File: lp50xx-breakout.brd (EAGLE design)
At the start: 31.8 x 29.2 mm, 17 parts, among them U1 LP5024

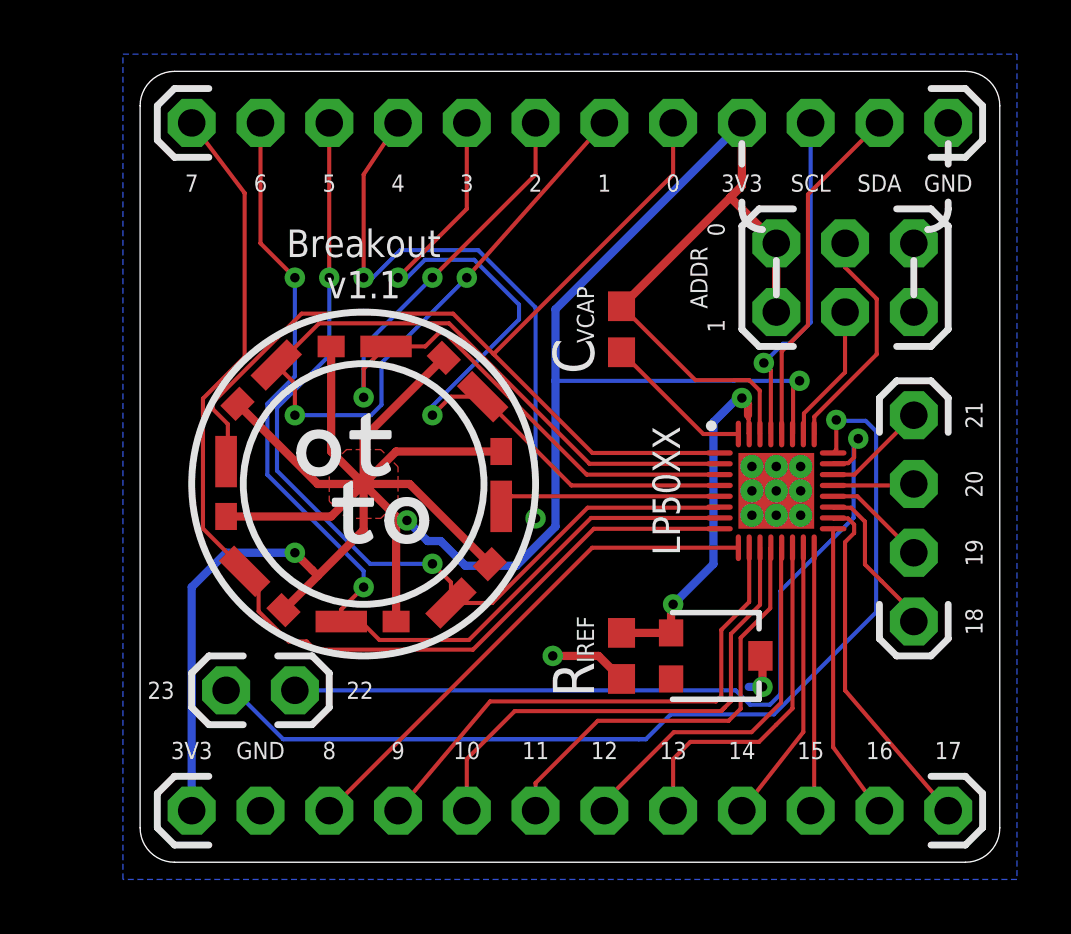
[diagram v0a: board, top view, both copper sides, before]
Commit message: Update design
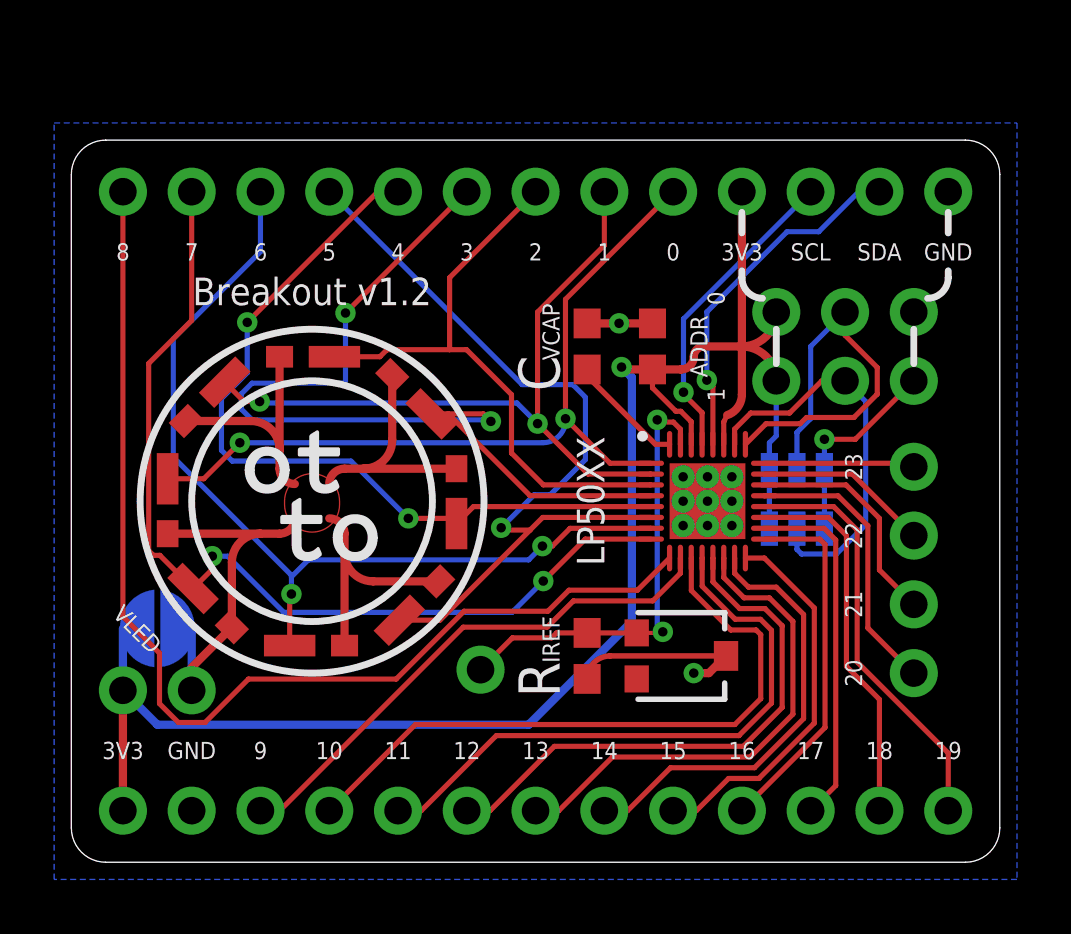
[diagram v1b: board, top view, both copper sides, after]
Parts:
- added C1: 1.0uF, SparkFun-Capacitors:0603
- added JP6: JUMPER-SMT_2_NO_NO-SILK_ROUND, SparkFun-Jumpers:SMT-JUMPER_2_NO_NO-SILK_ROUND
- added JP7, JP8: JUMPER-SMT_3_NO_NO_SILK, SparkFun-Jumpers:SMT-JUMPER_3_0-NO_TRACE_NO-SILK
- added JP9: (no value), pinhead-otto:1X01
- D1, D2, D3, D4, D5, D6, D7, D8: value (none) -> White, 60mA
- JP1, JP2: device pinhead-otto:1X12 -> pinhead-otto:1X13
- moved JP5 3.81 mm to (0.64, 6.35)
- moved JP1 2.84 mm to (14.6, 24.8)
- moved U1 2.57 mm to (21.0, 13.3)
- moved JP3 2.54 mm to (26.0, 19.1)
- moved D1 2.25 mm to (1.02, 13.3)
- moved D7 2.10 mm to (6.35, 8.00)
- moved D2 2.01 mm to (2.54, 17.1)
- moved D4 2.01 mm to (10.2, 17.1)
- moved D8 2.01 mm to (2.54, 9.53)
- moved D6 2.01 mm to (10.2, 9.53)
- moved D3 1.94 mm to (6.35, 18.7)
- moved JP4 1.90 mm to (28.6, 10.8), turned to 270 degrees
- moved D5 1.77 mm to (11.7, 13.3)
- moved C_VCAP 1.42 mm to (16.5, 19.1)
- moved JP2 1.27 mm to (14.6, 1.91)
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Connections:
- net N$5 renamed VCAP
- removed net N$1: R_IREF.2, U1.31, VR1.1
- new net IREF: JP9.1, R_IREF.2, U1.31, VR1.1
- new net VCC: D1.A, D2.A, D3.A, D4.A, D5.A, D6.A, D7.A, D8.A, JP5.1, JP6.2
- net +3V3: now also C1.1, JP5.2, JP6.1, JP7.3, JP8.1; no longer C_VCAP.1, D1.A, D2.A, D3.A, D4.A, D5.A, D6.A, D7.A, D8.A
- net ADDR0: now also JP8.2
- net ADDR1: now also JP7.2
- net GND: now also C1.2, C_VCAP.1, JP7.1, JP8.3
- net OUT10: now also JP2.4; no longer JP2.5
- net OUT11: now also JP2.5; no longer JP2.6
- net OUT12: now also JP2.6; no longer JP2.7
- net OUT13: now also JP2.7; no longer JP2.8
- net OUT14: now also JP2.8; no longer JP2.9
- net OUT15: now also JP2.9; no longer JP2.10
- net OUT16: now also JP2.10; no longer JP2.11
- net OUT17: now also JP2.11; no longer JP2.12
- net OUT18: now also JP2.12; no longer JP4.1
- net OUT19: now also JP2.13; no longer JP4.2
- net OUT20: now also JP4.4; no longer JP4.3
- net OUT21: now also JP4.3; no longer JP4.4
- net OUT22: now also JP4.2; no longer JP5.1
- net OUT23: now also JP4.1; no longer JP5.2
- net OUT8: now also JP1.13; no longer JP2.3
- net OUT9: now also JP2.3; no longer JP2.4
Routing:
- net +3V3: track 117.3 -> 66.7 mm, vias 3 -> 1
- net OUT23: track 49.7 -> 5.57 mm, vias 1 -> 0
- net VCC: track 0.00 -> 40.5 mm
- net OUT22: track 30.6 -> 6.46 mm, vias 1 -> 0
- net OUT8: track 19.1 -> 41.1 mm
- net IREF: track 0.00 -> 16.8 mm, vias 0 -> 2
- net N$1: track 13.1 -> 0.00 mm, vias 2 -> 0
- net GND: track 4.58 -> 16.9 mm, vias 2 -> 3
- net OUT19: track 3.84 -> 15.5 mm
- net OUT1: track 38.3 -> 26.8 mm
- net ADDR1: track 5.14 -> 15.2 mm
- net OUT18: track 5.83 -> 14.0 mm
- net OUT20: track 3.00 -> 10.4 mm
- net ADDR0: track 8.49 -> 15.7 mm
- net OUT2: track 29.7 -> 22.5 mm, vias 2 -> 0
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- added copper zone on layer 1, net VCC
- removed copper zone on layer 1, net +3V3
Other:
- board size 31.8 x 29.2 mm -> 34.3 x 26.7 mm
- board text added: "Breakout v1.2"
- board text added: "VLED"
- board text removed: "Breakout v1.1"
